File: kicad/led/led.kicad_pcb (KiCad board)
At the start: 2 copper layers, 123.8 x 88.9 mm, 85 parts, among them J1 Conn_01x09_Male, J2 Conn_01x09_Male, J3 Conn_01x09_Male, J4 Conn_01x09_Male, J5 Conn_01x09_Male

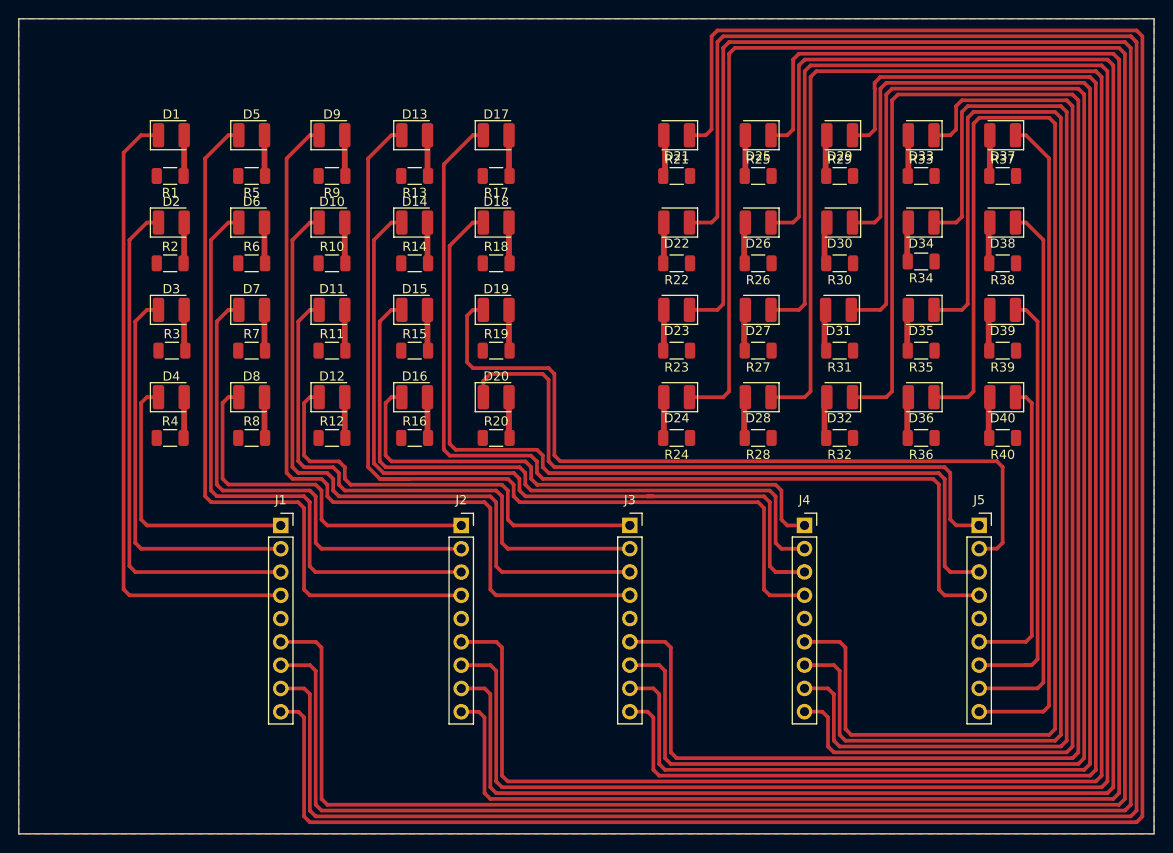
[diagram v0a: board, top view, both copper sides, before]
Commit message: Made some PCBs
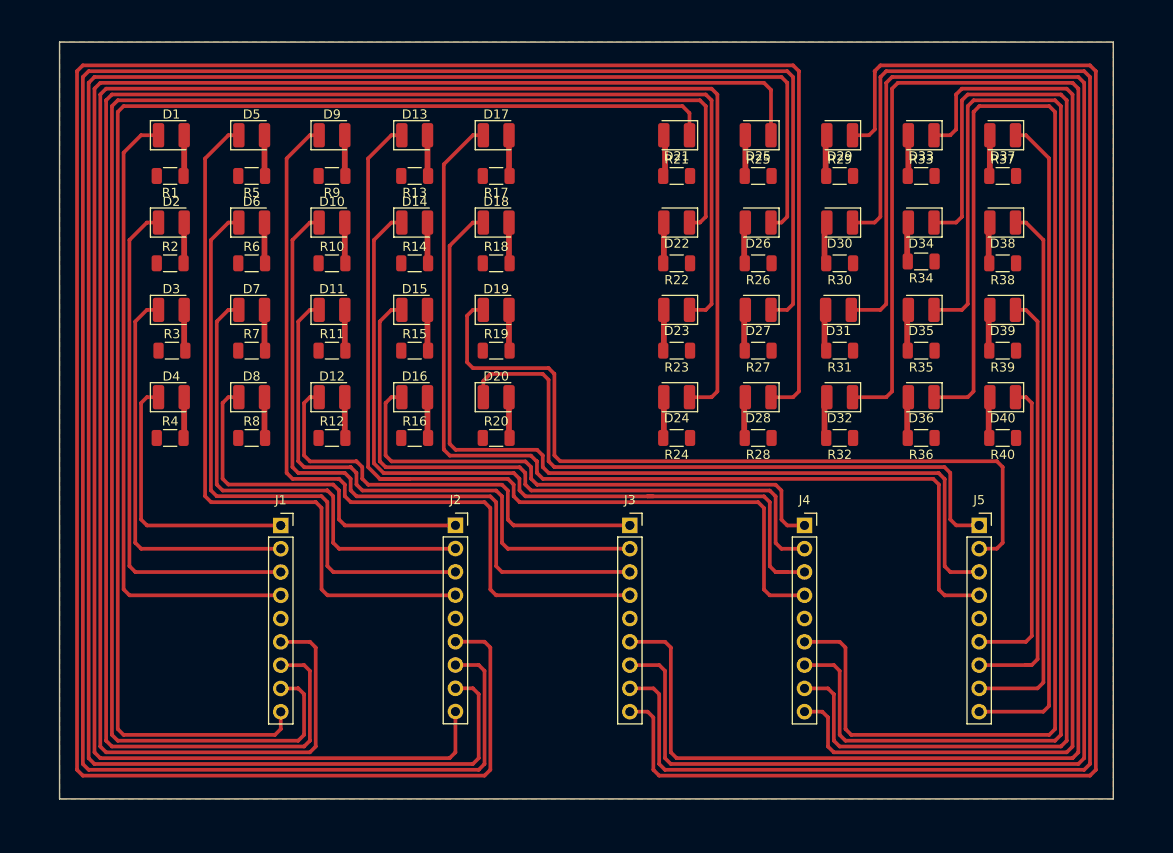
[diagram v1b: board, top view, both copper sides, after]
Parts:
- moved J2 0.64 mm to (78.7, 82.5)
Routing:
- net Net-(D21-Pad1): track 251.0 -> 152.9 mm
- net Net-(D22-Pad1): track 259.2 -> 176.7 mm
- net Net-(D23-Pad1): track 267.5 -> 195.1 mm
- net Net-(D24-Pad1): track 275.8 -> 213.5 mm
- net Net-(D28-Pad1): track 231.9 -> 256.7 mm
- net Net-(D27-Pad1): track 223.7 -> 238.3 mm
- net Net-(D25-Pad1): track 207.2 -> 196.1 mm
- net Net-(D26-Pad1): track 215.4 -> 219.9 mm
- net Net-(D35-Pad1): track 138.0 -> 140.5 mm
- net Net-(D30-Pad1): track 172.9 -> 175.5 mm
- net Net-(D29-Pad1): track 164.7 -> 167.2 mm
- net Net-(D36-Pad1): track 146.2 -> 148.8 mm
- net Net-(D33-Pad1): track 121.5 -> 124.0 mm
- net Net-(D32-Pad1): track 189.4 -> 192.0 mm
- net Net-(D31-Pad1): track 181.3 -> 183.8 mm
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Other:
- board size 123.8 x 88.9 mm -> 114.9 x 82.5 mm
